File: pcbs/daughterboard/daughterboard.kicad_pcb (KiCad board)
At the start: 2 copper layers, 33.5 x 18 mm, 5 parts, among them J1 Conn_01x10_Socket, U1 nice_nano

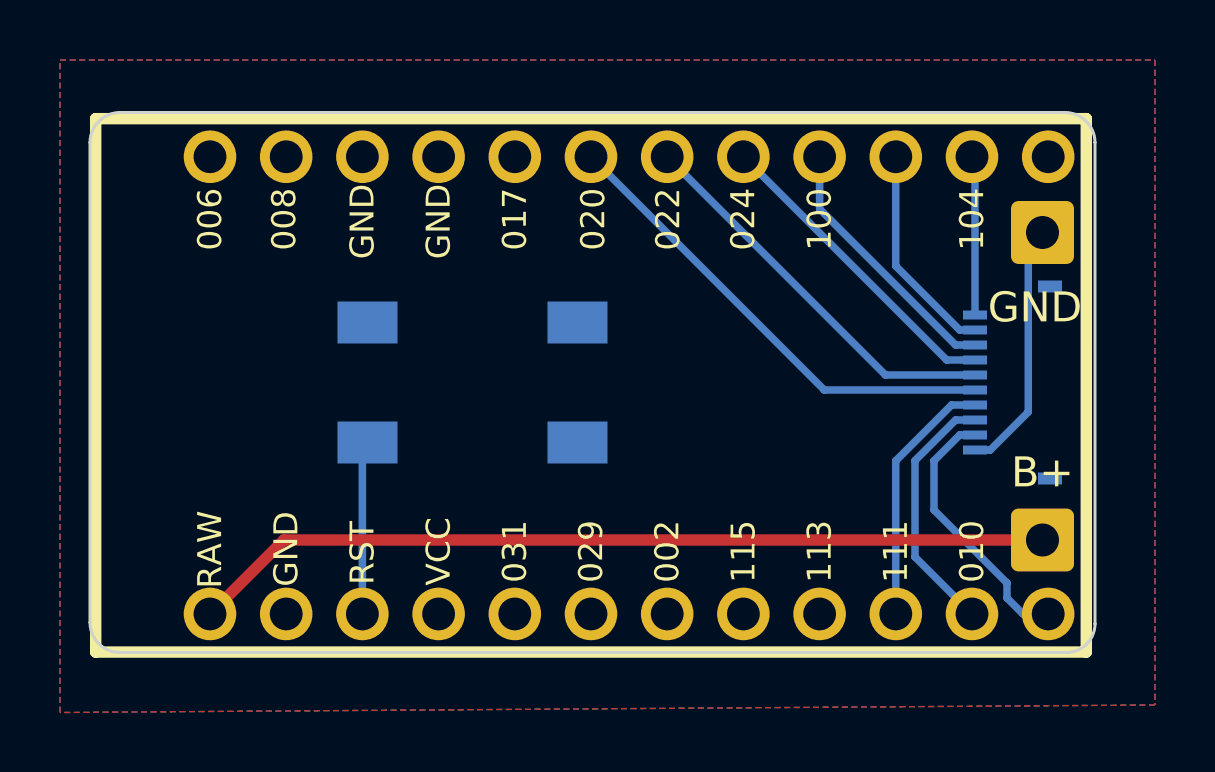
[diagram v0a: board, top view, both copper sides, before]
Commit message: plate and pcb finished
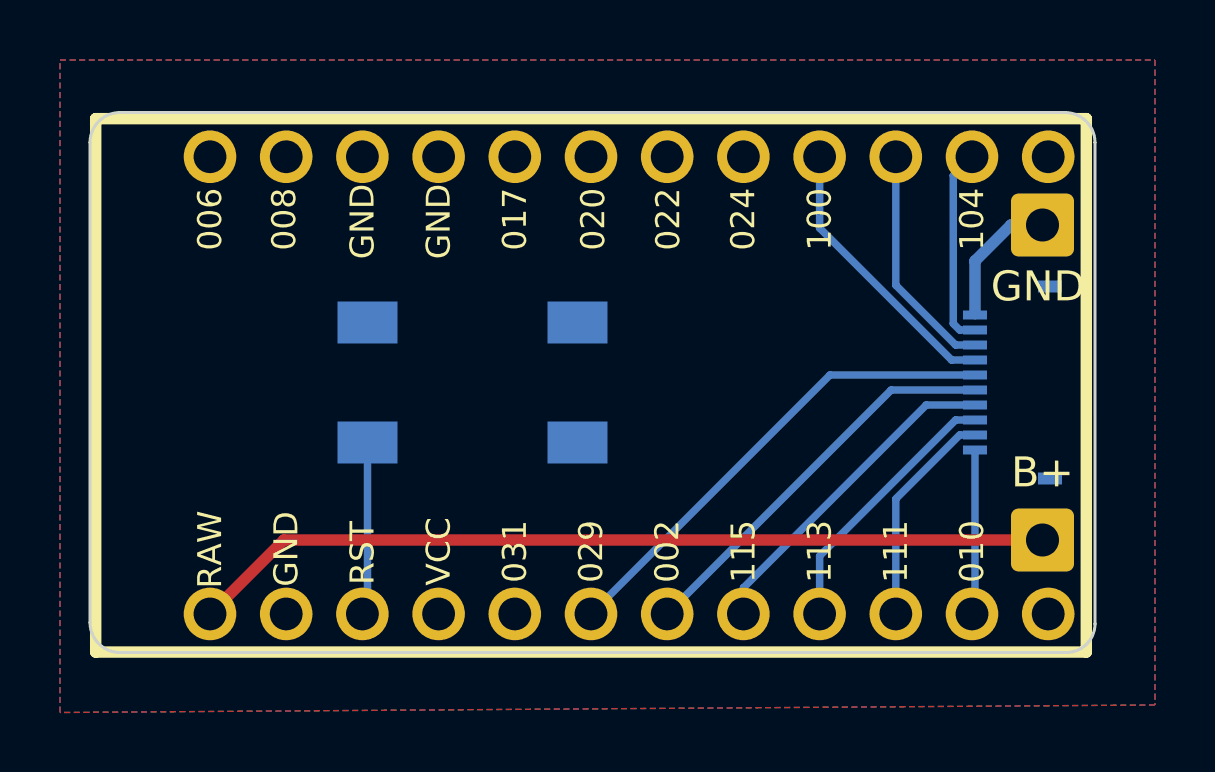
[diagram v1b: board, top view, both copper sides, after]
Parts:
- added G***: LOGO, art:baby_badger, B.Cu at (122.8, 109.0)
- B+: value Conn_01x01 -> B+
- moved GND 0.25 mm to (131.8, 103.8)
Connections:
- J1 pad 1: Column1 -> GND
- J1 pad 10: GND -> Column6
- J1 pad 2: Column2 -> Row1
- J1 pad 3: Column3 -> Row2
- J1 pad 4: Column4 -> Row3
- J1 pad 5: Column5 -> Column1
- J1 pad 6: Column6 -> Column2
- J1 pad 7: Row3 -> Column3
- J1 pad 8: Row2 -> Column4
- J1 pad 9: Row1 -> Column5
- U1 pad 10: Column2 -> Row2
- U1 pad 11: Column1 -> Row1
- U1 pad 13: Row1 -> unconnected-(U1-NFC1/P0.09-Pad13)
- U1 pad 14: Row2 -> Column6
- U1 pad 15: Row3 -> Column5
- U1 pad 16: Row4 -> Column4
- U1 pad 17: Row5 -> Column3
- U1 pad 18: Row6 -> Column2
- U1 pad 19: Row7 -> Column1
- U1 pad 20: Row8 -> unconnected-(U1-AIN7/P0.31-Pad20)
- U1 pad 5: Column7 -> unconnected-(U1-P0.17-Pad5)
- U1 pad 6: Column6 -> unconnected-(U1-P0.20-Pad6)
- U1 pad 7: Column5 -> unconnected-(U1-P0.22-Pad7)
- U1 pad 8: Column4 -> unconnected-(U1-P0.24-Pad8)
- U1 pad 9: Column3 -> Row3
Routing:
- net Column1: track 5.32 -> 16.1 mm
- net Column6: track 16.0 -> 5.51 mm
- net Column2: track 7.17 -> 13.4 mm
- net Column5: track 13.3 -> 7.36 mm
- net GND: track 8.48 -> 4.51 mm
- net Column3: track 8.80 -> 11.1 mm
- net Row1: track 8.90 -> 6.63 mm
- net Column4: track 10.5 -> 8.99 mm
- net Row3: track 8.52 -> 9.38 mm
- net Row2: track 8.46 -> 7.75 mm
